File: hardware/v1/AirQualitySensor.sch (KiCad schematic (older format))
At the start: 4 parts, among them U1 004-0-0053, U2 DHT22

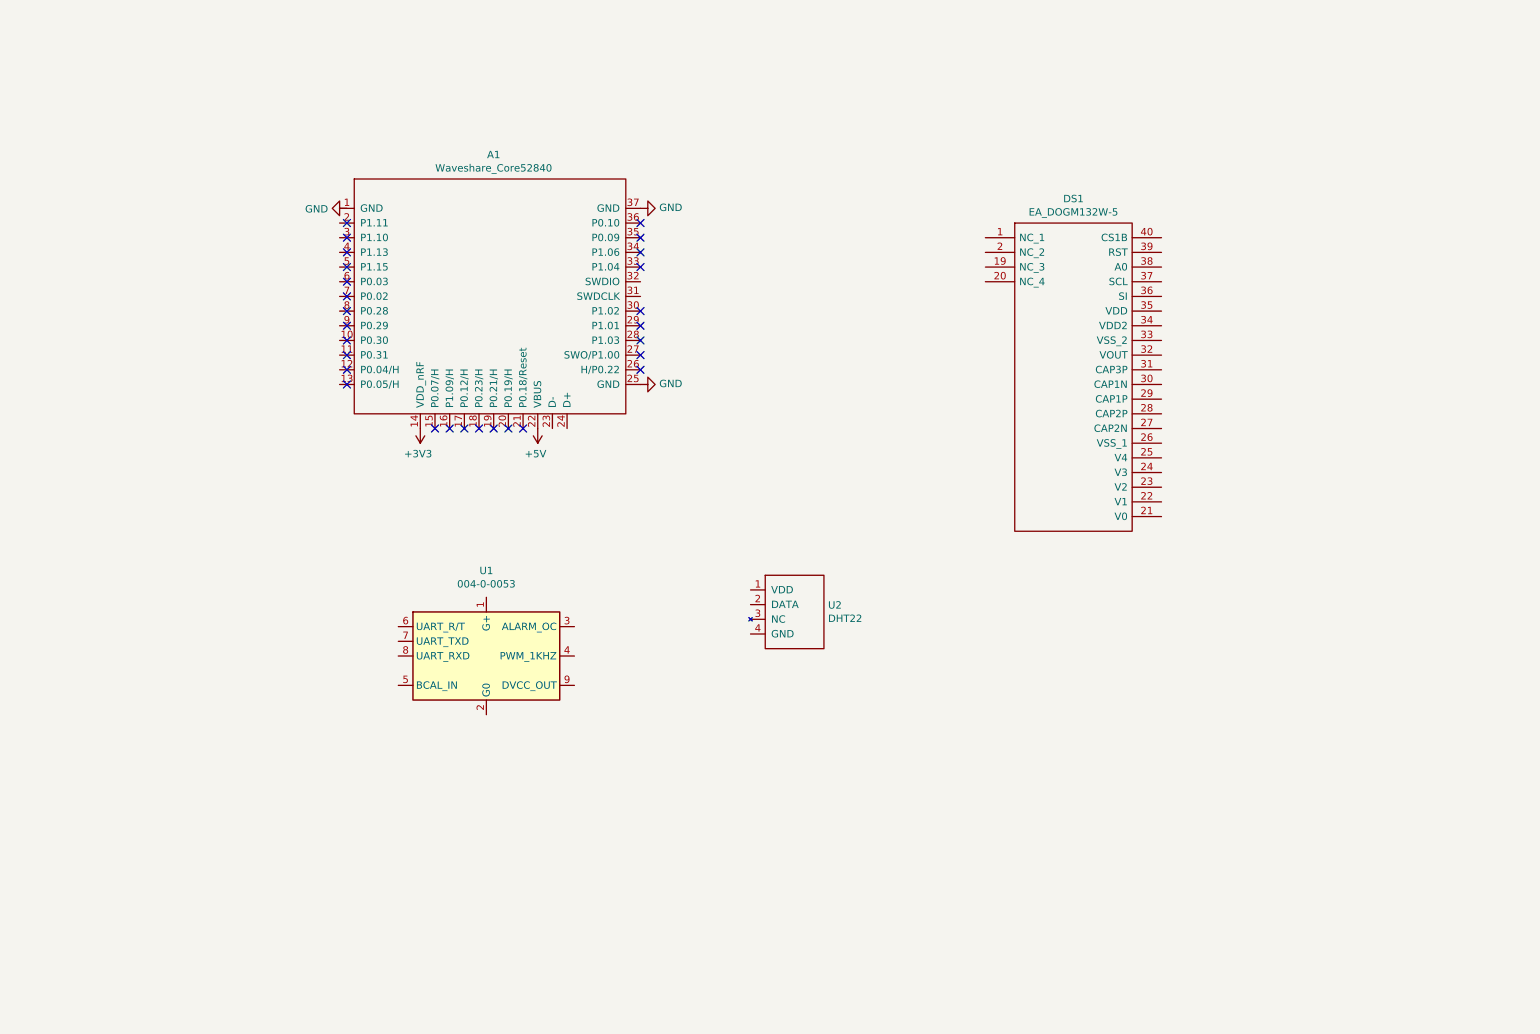
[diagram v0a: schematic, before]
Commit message: More Layout work
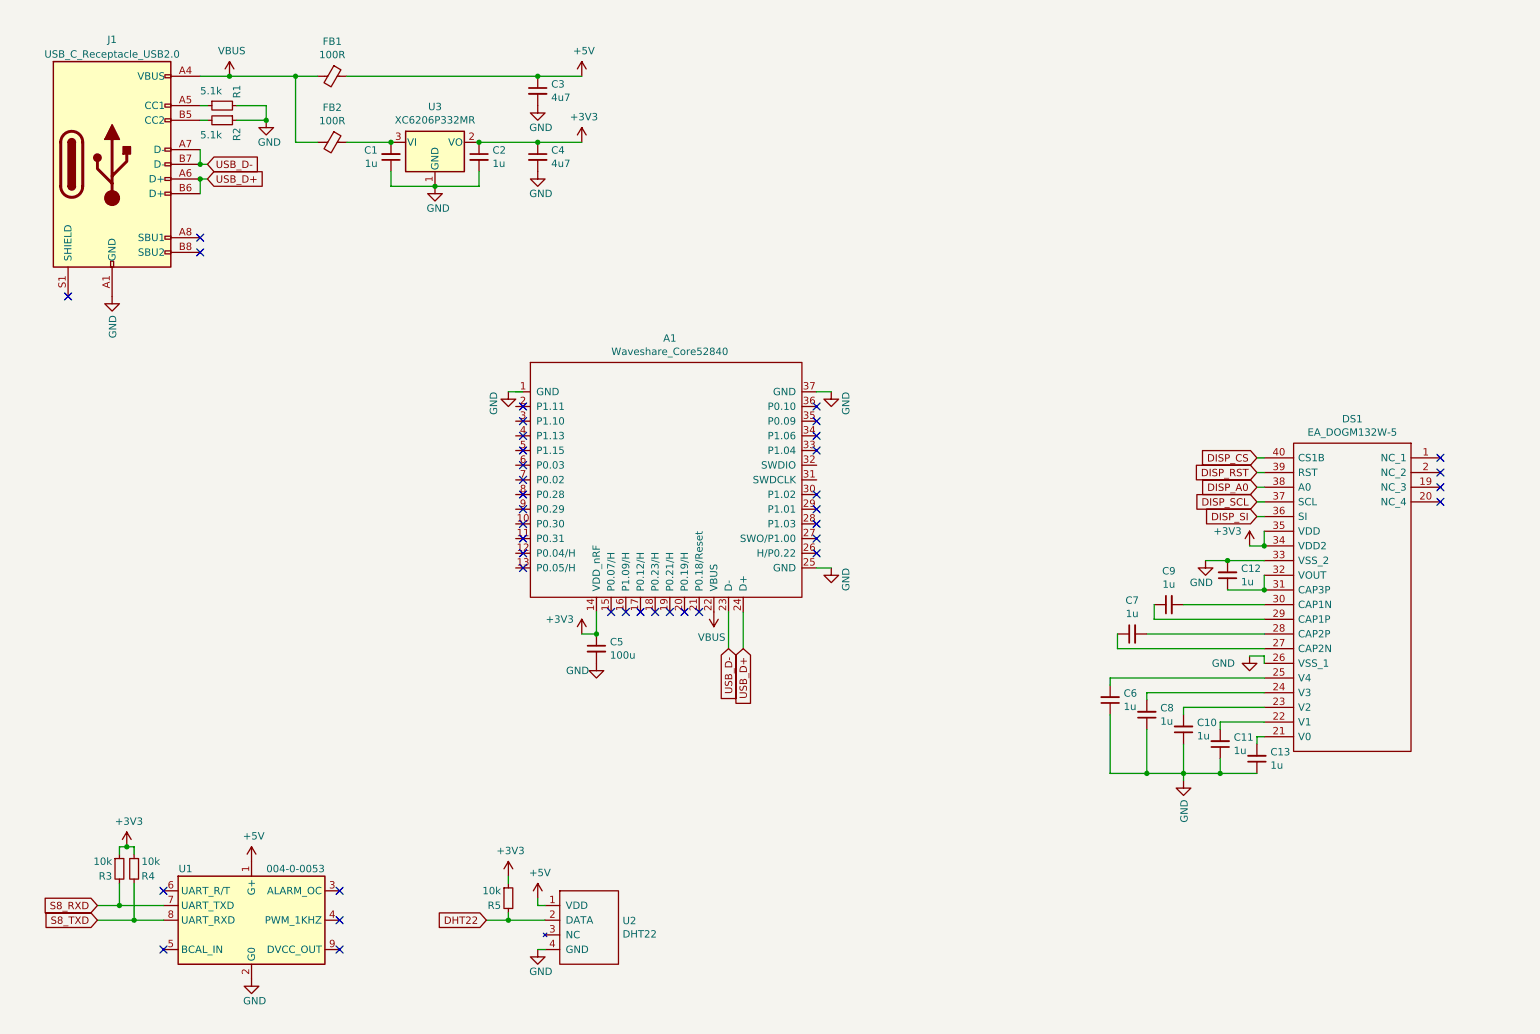
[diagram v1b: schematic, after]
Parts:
- added C1, C2: 1u, Capacitor_SMD:C_0603_1608Metric, symbol Device:C_Small
- added C10, C11, C12, C13, C6, C7, C8, C9: 1u, Capacitor_SMD:C_0402_1005Metric, symbol Device:C_Small
- added C3, C4: 4u7, Capacitor_SMD:C_0603_1608Metric, symbol Device:C_Small
- added C5: 100u, Capacitor_SMD:C_0402_1005Metric, symbol Device:C_Small
- added FB1, FB2: 100R, Inductor_SMD:L_0603_1608Metric, symbol Device:Ferrite_Bead_Small
- added J1: USB_C_Receptacle_USB2.0, Connector_USB:USB_C_Receptacle_HRO_TYPE-C-31-M-12, symbol Connector:USB_C_Receptacle_USB2.0
- added R1, R2: 5.1k, Resistor_SMD:R_0402_1005Metric, symbol Device:R_Small
- added R3, R4, R5: 10k, Resistor_SMD:R_0402_1005Metric, symbol Device:R_Small
- added U3: XC6206P332MR, Package_TO_SOT_SMD:SOT-23, symbol Regulator_Linear:XC6206PxxxMR
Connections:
- net +3V3: now also DS1.34 (VDD2), DS1.35 (VDD), C2.1, C4.1, C5.1, R3.1, R4.1, R5.1, U3.2 (VO)
- net +5V: now also U1.1 (G+), U2.1 (VDD), C3.1, FB1.1; no longer A1.22 (VBUS)
- net GND: now also DS1.26 (VSS_1), DS1.33 (VSS_2), U1.2 (G0), U2.4 (GND), C1.1, C10.1, C11.1, C12.2, C13.1, C2.2, C3.2, C4.2, C5.2, C6.1, C8.1, J1.A1 (GND), J1.A12 (GND), J1.B1 (GND), J1.B12 (GND), R1.2, R2.1, U3.1 (GND)
- net USB_D-: now reaches A1.23 (D-)
- net USB_D-: now also J1.A7 (D-), J1.B7 (D-)
- net USB_D+: now reaches A1.24 (D+)
- net USB_D+: now also J1.A6 (D+), J1.B6 (D+)
- net at DS1.21 (V0): now also C13.2
- net at DS1.22 (V1): now also C11.2
- net at DS1.23 (V2): now also C10.2
- net at DS1.24 (V3): now also C8.2
- net at DS1.25 (V4): now also C6.2
- net at DS1.27 (CAP2N): now also C7.1
- net at DS1.28 (CAP2P): now also C7.2
- net at DS1.29 (CAP1P): now also C9.1
- net at DS1.30 (CAP1N): now also C9.2
- net at DS1.31 (CAP3P): now also DS1.32 (VOUT), C12.1
- net DISP_SI: now reaches DS1.36 (SI)
- net DISP_SCL: now reaches DS1.37 (SCL)
- net DISP_A0: now reaches DS1.38 (A0)
- net DISP_RST: now reaches DS1.39 (RST)
- net DISP_CS: now reaches DS1.40 (CS1B)
- net S8_RXD: now reaches U1.7 (UART_TXD)
- net S8_RXD: now also R3.2
- net S8_TXD: now reaches U1.8 (UART_RXD)
- net S8_TXD: now also R4.2
- net DHT22: now reaches U2.2 (DATA)
- net DHT22: now also R5.2
- new net: J1.A5 (CC1), R1.1
- new net: J1.B5 (CC2), R2.2
- new net: C1.2, FB2.1, U3.3 (VI)
- new net VBUS: A1.22 (VBUS), FB1.2, FB2.2, J1.A4 (VBUS), J1.A9 (VBUS), J1.B4 (VBUS), J1.B9 (VBUS)
- no-connect marks 28 -> 40
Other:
- moved on the sheet: A1, DS1, U1, U2

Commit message: Continue schematic
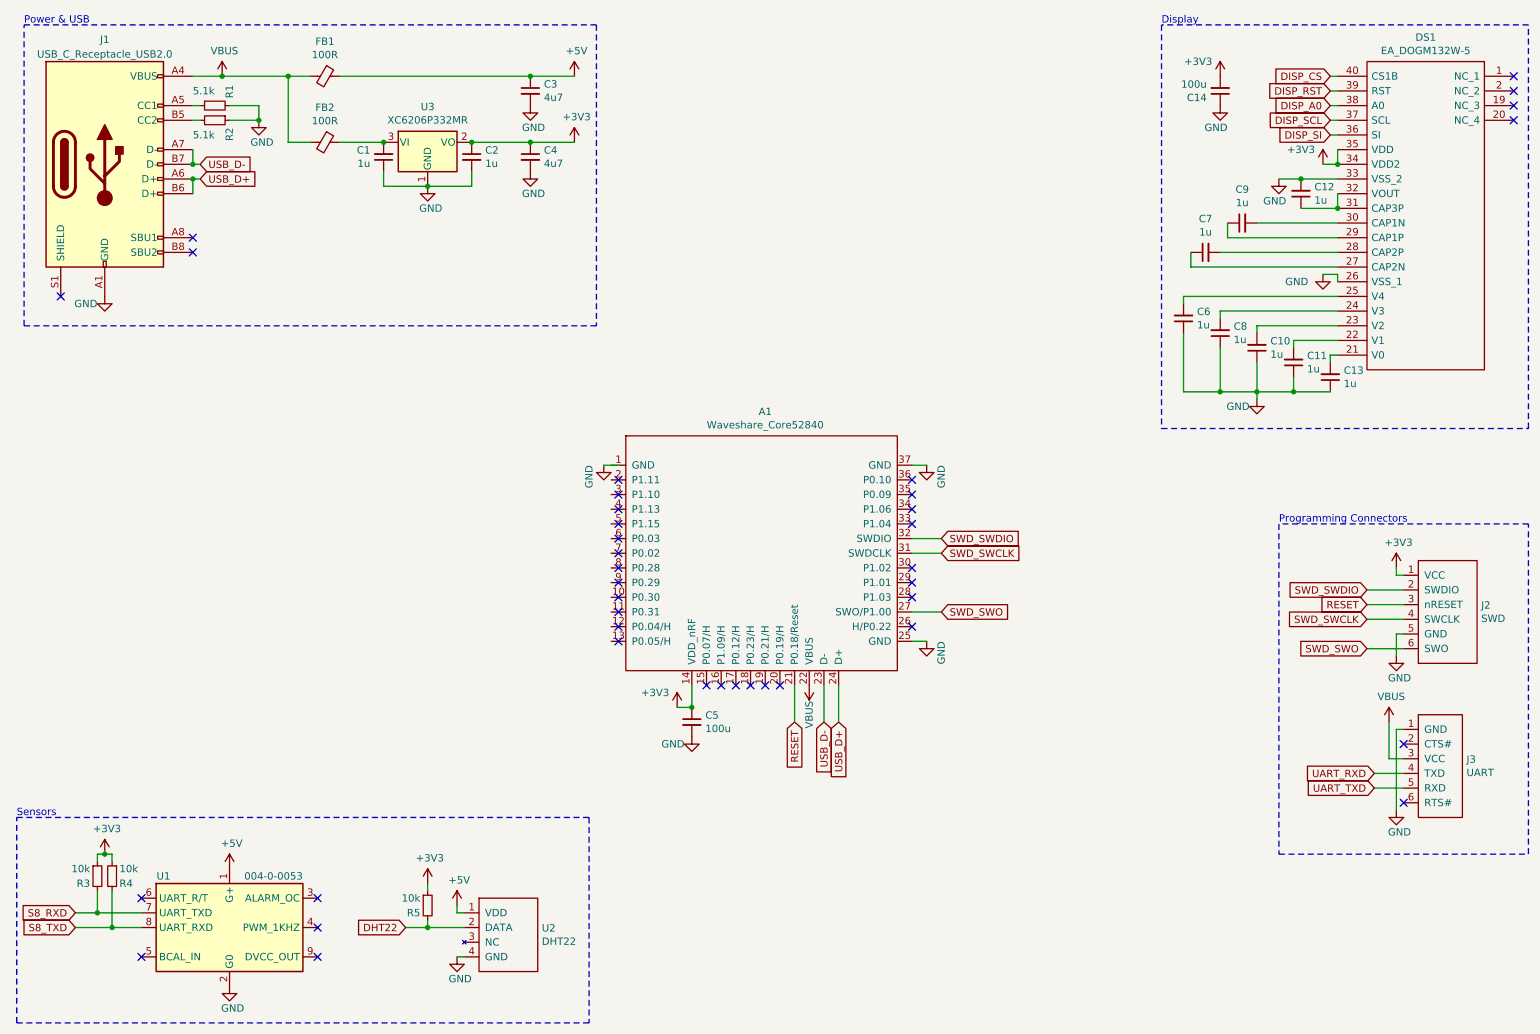
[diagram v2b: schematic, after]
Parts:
- added C14: 100u, Capacitor_SMD:C_0402_1005Metric, symbol Device:C_Small
- added J2: SWD, AirQualitySensor:TC2030-IDC-FP, symbol AirQualitySensor:TC2030
- added J3: UART, Connector_PinHeader_2.54mm:PinHeader_1x06_P2.54mm_Vertical, symbol AirQualitySensor:UART_ftdi
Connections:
- net +3V3: now also C14.2, J2.1 (VCC)
- net GND: now also C14.1, J2.5 (GND), J3.1 (GND)
- net VBUS: now also J3.3 (VCC)
- net RESET: now reaches A1.21 (P0.18/Reset)
- net RESET: now also J2.3 (nRESET)
- net SWD_SWO: now reaches A1.27 (SWO/P1.00)
- net SWD_SWO: now also J2.6 (SWO)
- net SWD_SWCLK: now reaches A1.31 (SWDCLK)
- net SWD_SWCLK: now also J2.4 (SWCLK)
- net SWD_SWDIO: now reaches A1.32 (SWDIO)
- net SWD_SWDIO: now also J2.2 (SWDIO)
- new net UART_RXD: J3.4 (TXD)
- new net UART_TXD: J3.5 (RXD)
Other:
- note added: "Display"
- note added: "Power & USB"
- note added: "Programming Connectors"
- note added: "Sensors"
- moved on the sheet: A1, C1, C10, C11, C12, C13, C2, C3, C4, C5, C6, C7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
